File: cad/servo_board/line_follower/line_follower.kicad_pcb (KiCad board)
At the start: 2 copper layers, 50 x 22 mm, 18 parts, among them J1 Conn_01x02, J2 Conn_01x02, J4 Servo Header x2, J6 Conn_01x02, J9 Conn_01x06_MountingPin, Q1 LOW PWR FET, Q2 LOW PWR FET

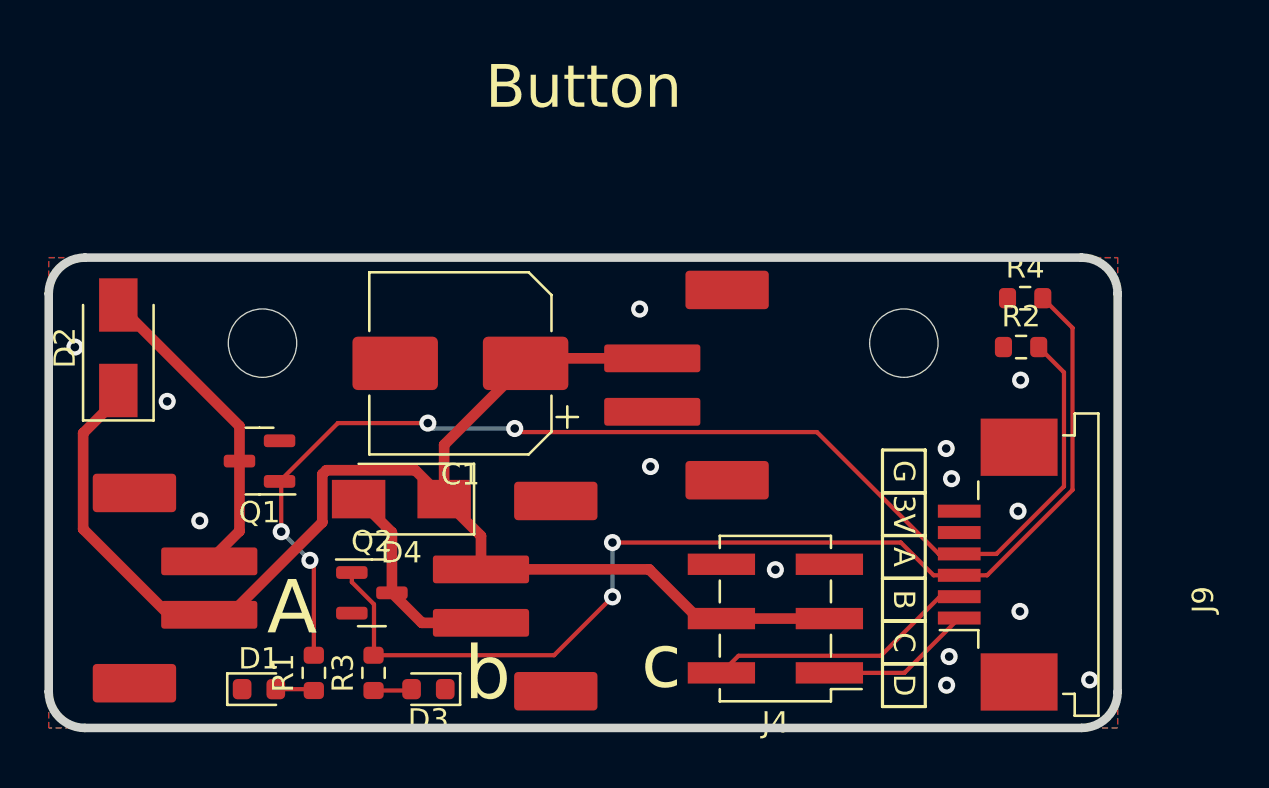
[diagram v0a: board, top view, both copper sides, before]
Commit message: tracey thingies
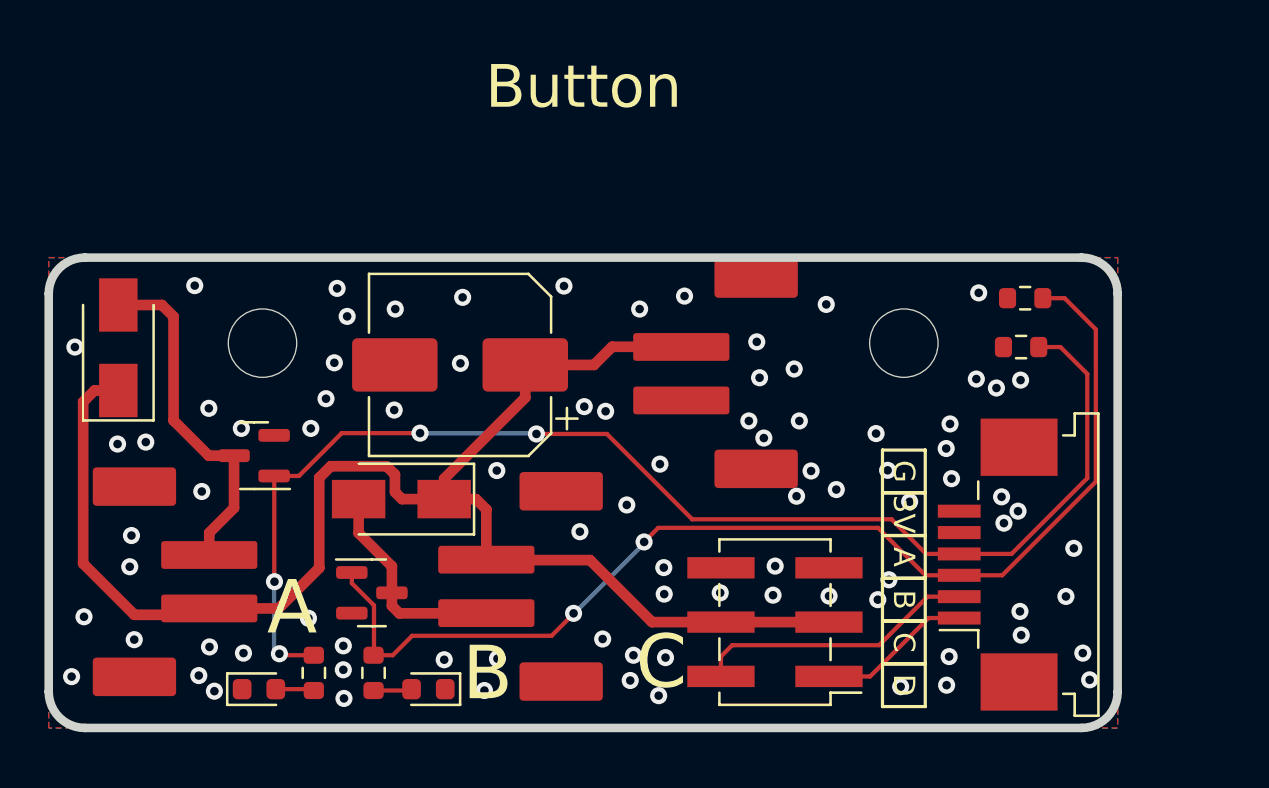
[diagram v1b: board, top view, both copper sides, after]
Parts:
- moved J6 1.46 mm to (174.8, 76.4)
- moved J2 0.52 mm to (165.7, 86.4)
- moved Q1 0.36 mm to (149.6, 80.3)
- moved J1 0.30 mm to (142.3, 86.2)
- moved J4 0.17 mm to (174.0, 88.0)
- moved C1 0.08 mm to (159.2, 76.0)
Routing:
- net +VDC: track 65.6 -> 71.0 mm
- net /Thing 1: track 57.5 -> 60.4 mm
- net Net-(D2-Pad2): track 14.9 -> 16.3 mm
- net /Thing 2: track 52.5 -> 53.6 mm
- net /SERVO_2: track 12.6 -> 13.2 mm
- net GND: vias 14 -> 86
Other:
- board text removed: "b"
- board text removed: "c"
